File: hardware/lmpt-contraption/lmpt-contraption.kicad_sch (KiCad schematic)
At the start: 22 parts, among them IC1 SN74LVC541APW, J1 CLK_IN, J2 CLK_A, J3 CLK_B, J4 1PPS Out Conn, J5 RPi Out Conn, U1 LT1117-3.3, U2 74LVC2G17

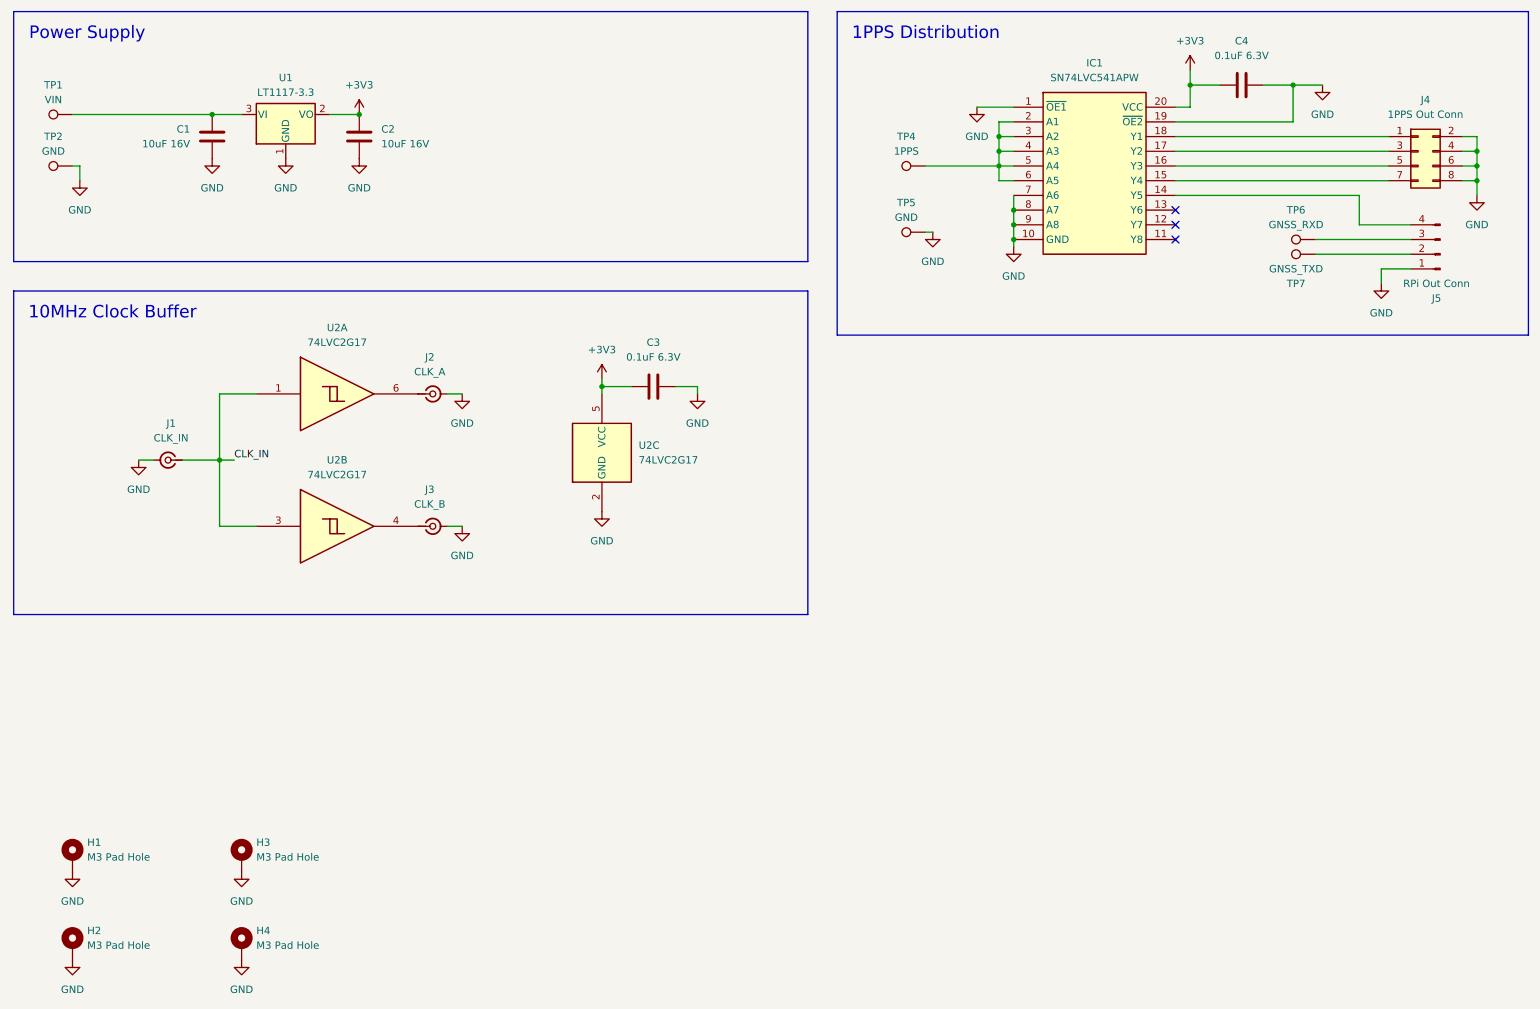
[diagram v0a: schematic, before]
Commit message: feat(LMPT-contraption): revision B
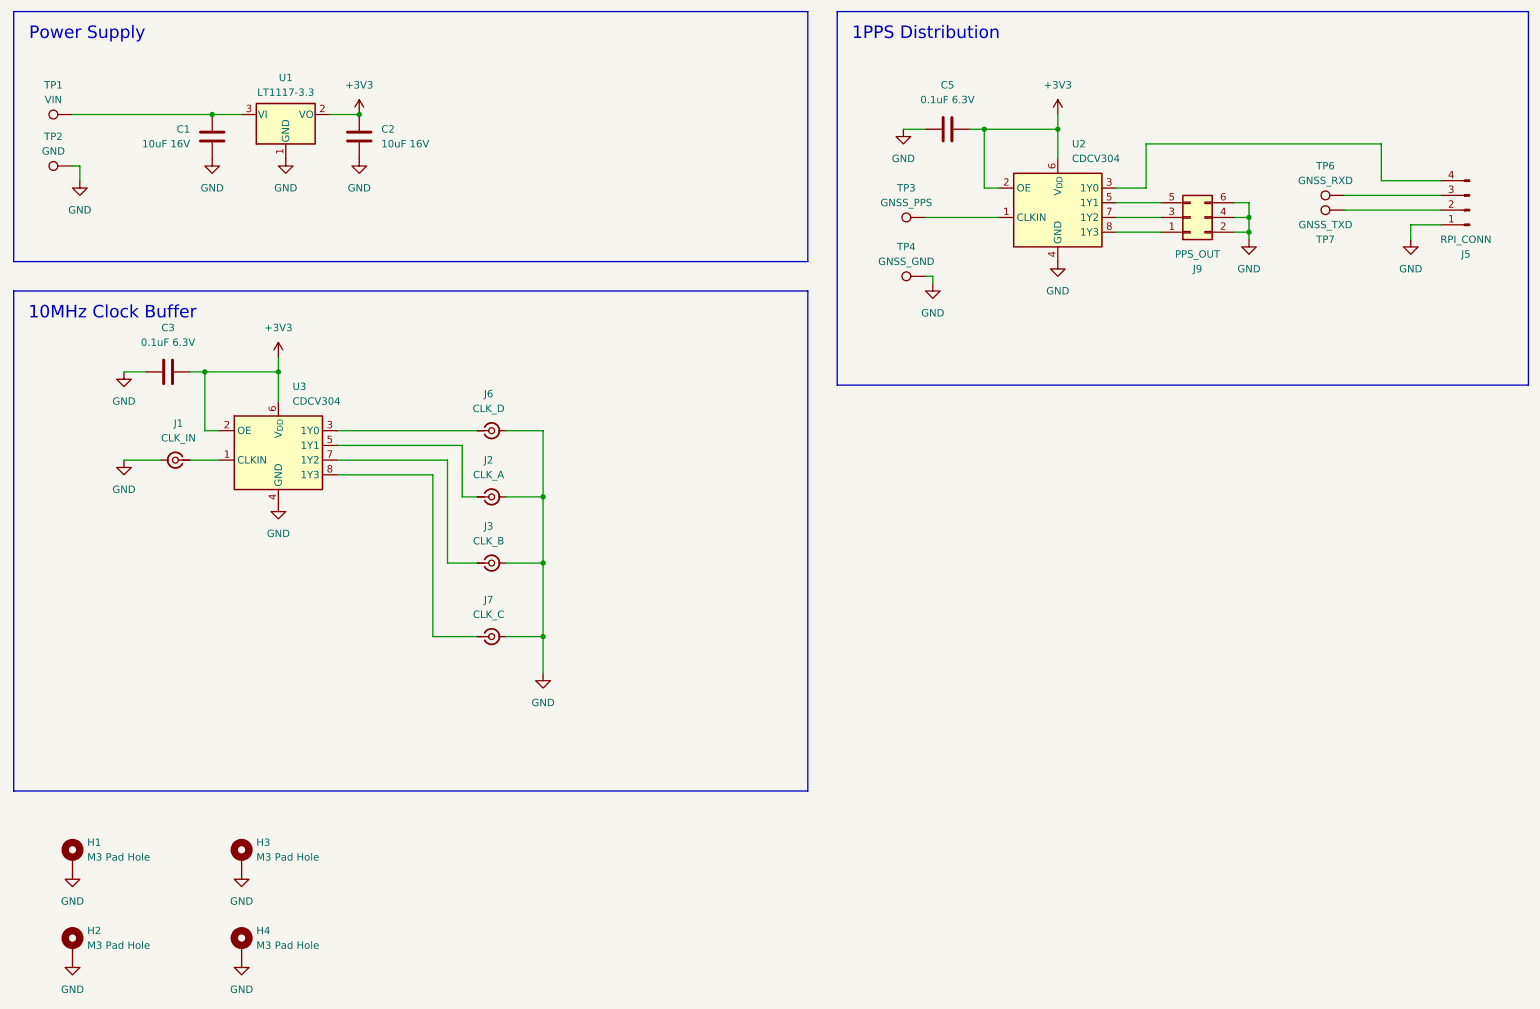
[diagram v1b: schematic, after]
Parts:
- removed C4: 0.1uF 6.3V, Capacitor_SMD:C_0805_2012Metric, symbol Device:C
- removed IC1: SN74LVC541APW, Package_SO:TSSOP-20_4.4x6.5mm_P0.65mm, symbol BKSP:Logic_SN74LVC541APW
- removed J4: 1PPS Out Conn, Connector_PinHeader_2.54mm:PinHeader_2x04_P2.54mm_Vertical_SMD, symbol Connector_Generic:Conn_02x04_Odd_Even
- removed TP5: GND, TestPoint:TestPoint_Pad_2.0x2.0mm, symbol Connector:TestPoint
- removed U2: 74LVC2G17, Package_TO_SOT_SMD:SOT-23-6, symbol 74xGxx:74LVC2G17
- added C5: 0.1uF 6.3V, Capacitor_SMD:C_0805_2012Metric, symbol Device:C
- added J6: CLK_D, Connector_Coaxial:U.FL_Molex_MCRF_73412-0110_Vertical, symbol Connector:Conn_Coaxial_Small
- added J7: CLK_C, Connector_Coaxial:U.FL_Molex_MCRF_73412-0110_Vertical, symbol Connector:Conn_Coaxial_Small
- added J9: PPS_OUT, Connector_PinHeader_2.54mm:PinHeader_2x03_P2.54mm_Vertical_SMD, symbol Connector_Generic:Conn_02x03_Odd_Even
- added TP3: GNSS_PPS, TestPoint:TestPoint_Pad_D2.0mm, symbol Connector:TestPoint
- added U2, U3: CDCV304, Package_SO:TSSOP-8_4.4x3mm_P0.65mm, symbol Buffer:CDCV304
- J2, J3: footprint Connector_Coaxial:U.FL_Molex_MCRF_73412-0110_Vertical -> Connector_Coaxial:SMA_Molex_73251-1153_EdgeMount_Horizontal
- J5: value RPi Out Conn -> RPI_CONN
- TP4: value 1PPS -> GNSS_GND; footprint TestPoint:TestPoint_Pad_D2.0mm -> TestPoint:TestPoint_Pad_2.0x2.0mm
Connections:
- net +3V3: now also C5.1, U2.2 (OE), U2.6 (V_{DD}), U3.2 (OE), U3.6 (V_{DD})
- net GND: now also TP4.1, C5.2, J6.2 (Ext), J7.2 (Ext), J9.2 (Pin_2), J9.4 (Pin_4), J9.6 (Pin_6), U2.4 (GND), U3.4 (GND)
- net at J2.1 (In): now also U3.5 (1Y1)
- net at J5.4 (Pin_4): now also U2.3 (1Y0)
- net at J3.1 (In): now also U3.7 (1Y2)
- net CLK_IN: no longer names the net of J1.1 (In)
- net CLK_IN: now also U3.1 (CLKIN)
- new net: TP3.1, U2.1 (CLKIN)
- new net: J9.1 (Pin_1), U2.8 (1Y3)
- new net: J9.3 (Pin_3), U2.7 (1Y2)
- new net: J9.5 (Pin_5), U2.5 (1Y1)
- new net: J7.1 (In), U3.8 (1Y3)
- new net: J6.1 (In), U3.3 (1Y0)
- no-connect marks 3 -> 0
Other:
- moved on the sheet: J1, J2, J3, J5, TP6, TP7
